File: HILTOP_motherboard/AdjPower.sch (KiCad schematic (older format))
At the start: 92 parts, among them Q1 Q_NMOS_DS_POWERPAK, Q2 Q_NMOS_DS_POWERPAK, Q4 2N7002, U10 TLC271, U11 ADS1015, U12 MCP4725, U8 LM5118, U9 INA250A3

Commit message: Schematics complete - 1st draft
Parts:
- C111, C112, C115, C117, C118, C179, C180, C181, C182, C183, C184, C185, C187, C188, C189, C190, C191, C192, C193, C194, C54, C56, C57, C58, C60, C61, C62, C63, C64, C65, C69: symbol C -> device:C
- C186, C67, C70, C79: symbol CP -> device:CP
- D10, D7, D8, D9: symbol D_x2_Serial_AKC -> device:D_x2_Serial_AKC
- D19: symbol D_Schottky -> device:D_Schottky
- D20: symbol D -> device:D
- D5: symbol D_Schottky_x2_KCom_AAK -> device:D_Schottky_x2_KCom_AAK
- D6: symbol D_Schottky_x2_KCom_AKA -> device:D_Schottky_x2_KCom_AKA
- L4: symbol L -> device:L
- Q1, Q2: symbol Q_NMOS_DS_POWERPAK -> Devtank:Q_NMOS_DS_POWERPAK
- Q4: symbol 2N7002 -> Transistor:2N7002
- R105, R112, R113, R114, R115, R116, R117, R118, R123, R132, R133, R142, R143, R165, R166, R57, R58, R59, R60, R61, R62, R63, R64, R65, R66, R67, R68, R69, R74, R75, R76: symbol R -> device:R
- RL1: symbol SPST-NO -> Devtank:SPST-NO
- TP1, TP2, TP3, TP4, TP5, TP6, TP7: footprint TestPoint:TestPoint_THTPad_D1.5mm_Drill0.7mm -> TestPoint:TestPoint_THTPad_D1.0mm_Drill0.5mm; symbol TEST_1P -> HILTOP_Motherboard-rescue:TEST_1P
- U10: symbol TLC271 -> Devtank:TLC271
- U11: symbol ADS1015 -> Devtank:ADS1015
- U12: symbol MCP4725 -> Devtank:MCP4725
- U8: symbol LM5118 -> Devtank:LM5118
- U9: symbol INA250 -> Devtank:INA250
- W1: symbol TEST_1P -> HILTOP_Motherboard-rescue:TEST_1P
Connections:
- net labels removed: PSU_ADC_ADDR, PSU_ALERT_RDY, PSU_DAC_ADDR
- wire segments 306 -> 418

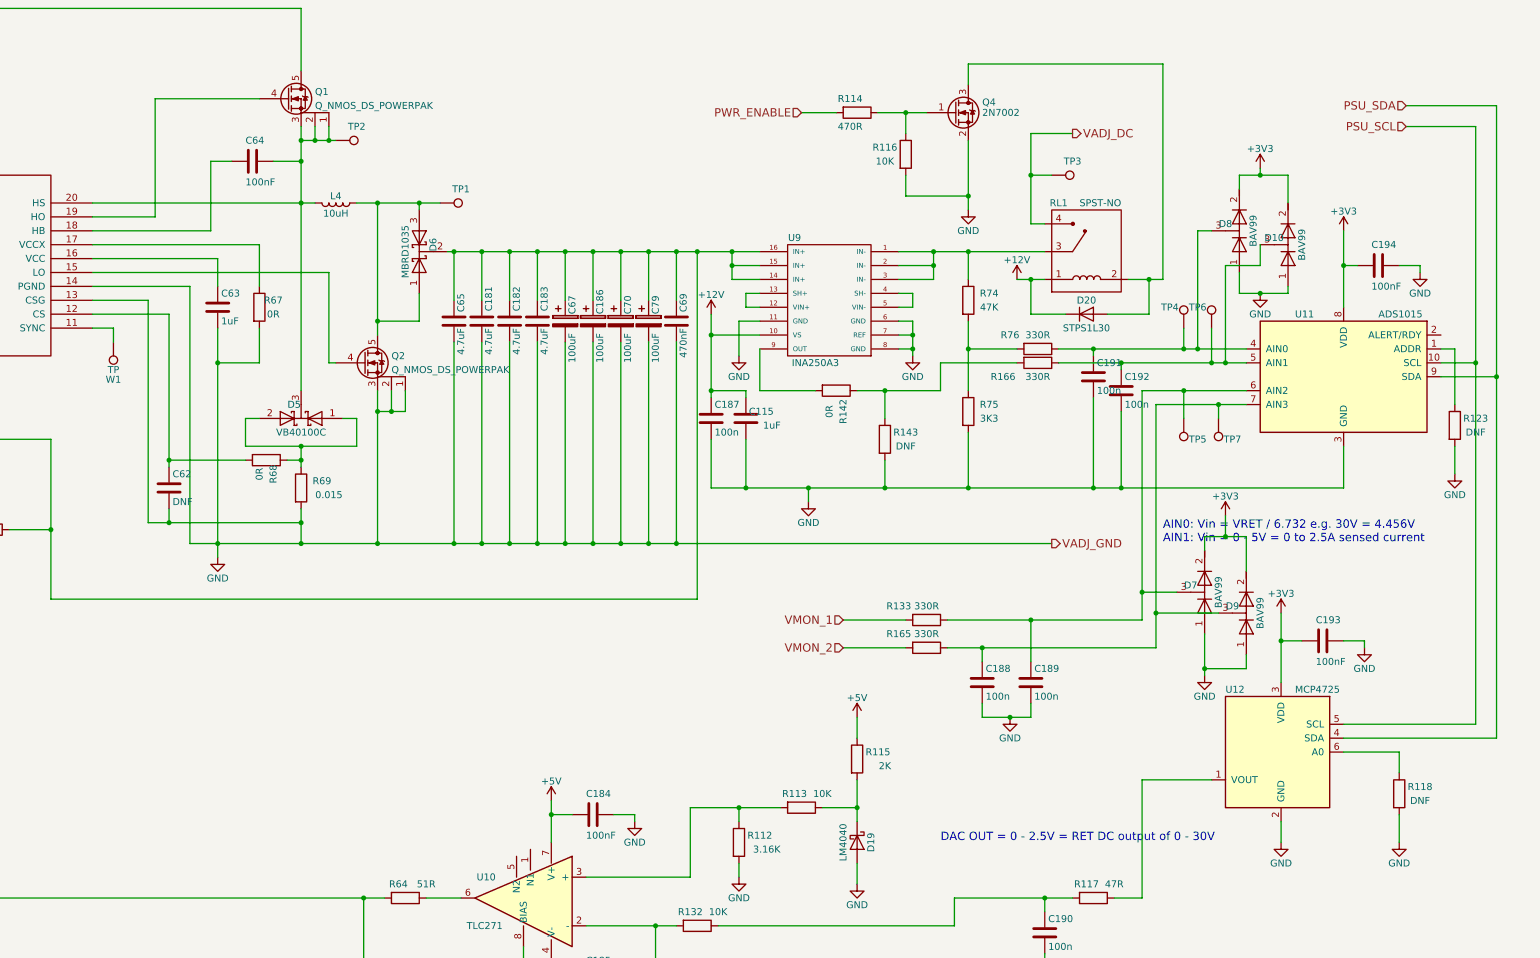
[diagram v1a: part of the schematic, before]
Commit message: BOM nearly complete!
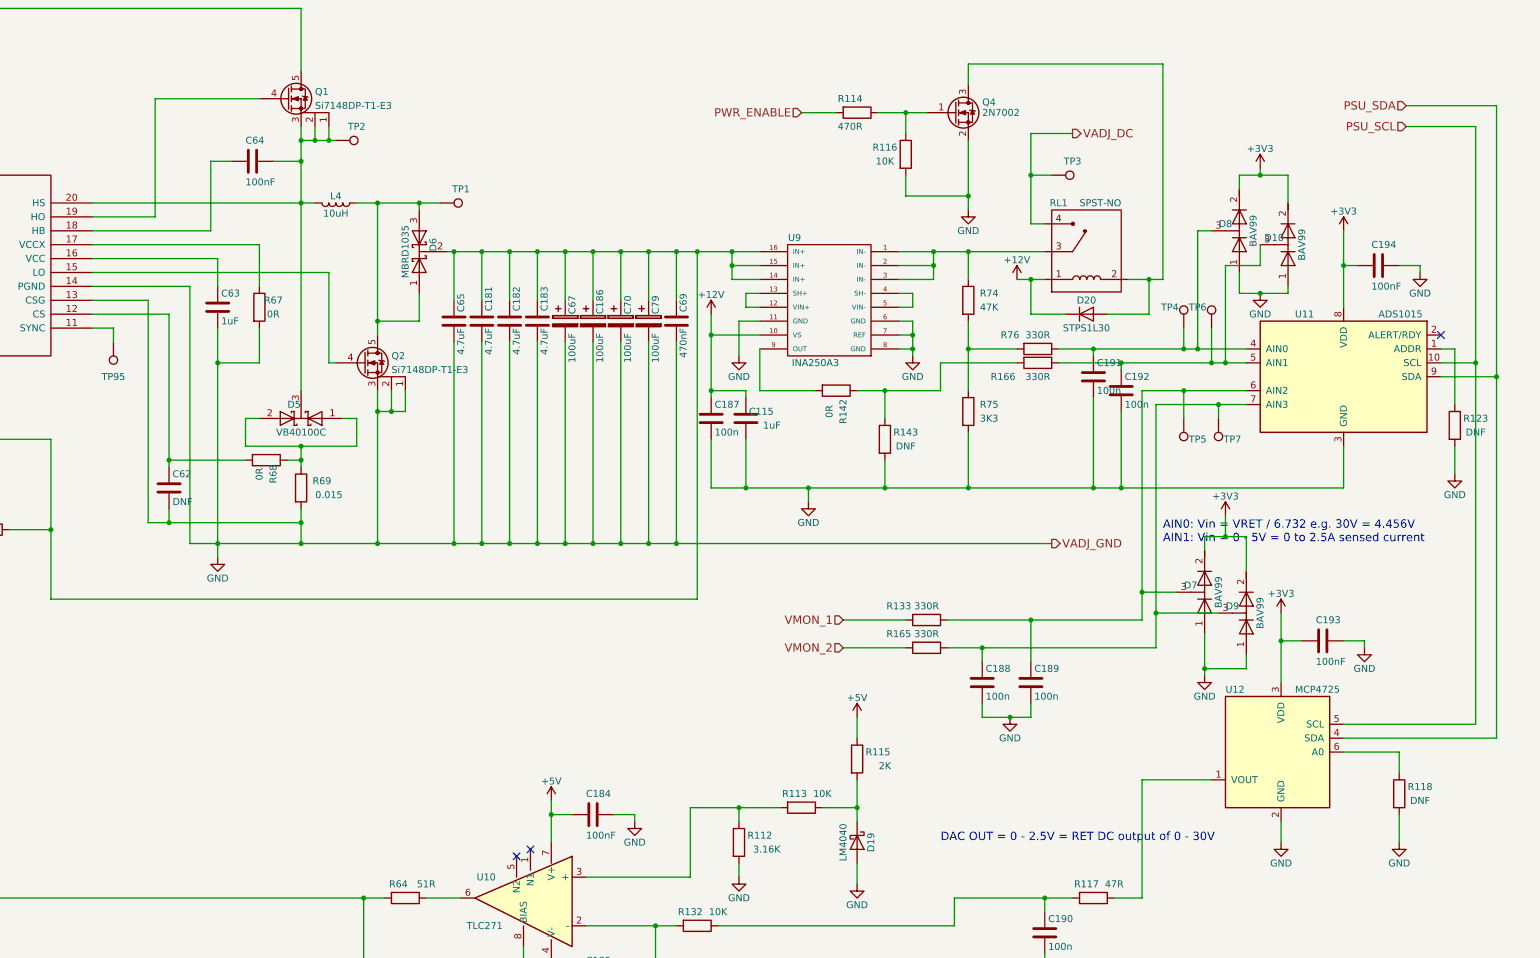
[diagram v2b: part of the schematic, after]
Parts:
- removed W1: TP, TestPoint:TestPoint_THTPad_1.5x1.5mm_Drill0.7mm, symbol HILTOP_Motherboard-rescue:TEST_1P
- added TP95: TP, TestPoint:TestPoint_THTPad_D1.0mm_Drill0.5mm, symbol HILTOP_Motherboard-rescue:TEST_1P
- Q1, Q2: value Q_NMOS_DS_POWERPAK -> Si7148DP-T1-E3
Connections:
- net at U8.11 (SYNC): now also TP95.1
- no-connect marks 0 -> 3
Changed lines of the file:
@@
 $Descr A3 16535 11693
 encoding utf-8
-Sheet 7 12
+Sheet 6 12
 Title "HILTOP Motherboard"
 Date "26th January 2018"
@@
 $EndComp
 $Comp
-L HILTOP_Motherboard-rescue:TEST_1P W1
-U 1 1 58E90AB1
-P 5550 4850
-F 0 "W1" H 5550 5120 50  0000 C CNN
-F 1 "TP" H 5550 5050 50  0000 C CNN
-F 2 "TestPoint:TestPoint_THTPad_1.5x1.5mm_Drill0.7mm" H 5750 4850 50  0001 C CNN
-F 3 "" H 5750 4850 50  0000 C CNN
-	1    5550 4850
-	-1   0    0    1
-$EndComp
-$Comp
 L device:C C64
 U 1 1 58E9153E
@@
 P 6800 3100
 F 0 "Q1" H 7000 3150 50  0000 L CNN
-F 1 "Q_NMOS_DS_POWERPAK" H 7000 3050 50  0000 L CNN
+F 1 "Si7148DP-T1-E3" H 7000 3050 50  0000 L CNN
 F 2 "Devtank_PCB_Lib:PowerPAK_SO-8" H 7000 3200 50  0001 C CNN
 F 3 "" H 6800 3100 50  0000 C CNN
@@
 P 7350 5000
 F 0 "Q2" H 7550 5050 50  0000 L CNN
-F 1 "Q_NMOS_DS_POWERPAK" H 7550 4950 50  0000 L CNN
+F 1 "Si7148DP-T1-E3" H 7550 4950 50  0000 L CNN
 F 2 "Devtank_PCB_Lib:PowerPAK_SO-8" H 7550 5100 50  0001 C CNN
 F 3 "" H 7350 5000 50  0000 C CNN
@@
 Wire Wire Line
 	9400 6300 9600 6300
+NoConn ~ 15100 4800
+NoConn ~ 8550 8500
+NoConn ~ 8450 8550
+$Comp
+L HILTOP_Motherboard-rescue:TEST_1P TP?
+U 1 1 5CBFAD8E
+P 5550 4850
+AR Path="/5CBFAD8E" Ref="TP?"  Part="1"
+AR Path="/589A1BA0/5CBFAD8E" Ref="TP95"  Part="1"
+F 0 "TP95" H 5550 5100 50  0000 C CNN
+F 1 "TP" H 5550 5050 50  0001 C CNN
+F 2 "TestPoint:TestPoint_THTPad_D1.0mm_Drill0.5mm" H 5750 4850 50  0001 C CNN
+F 3 "" H 5750 4850 50  0000 C CNN
+	1    5550 4850
+	-1   0    0    1
+$EndComp
 $EndSCHEMATC
